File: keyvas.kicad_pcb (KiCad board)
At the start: 2 copper layers, 133 parts, among them J2 SWD, J3 USB-C Conn, J4 Conn_01x02_Female, K1 KEYSW, K10 KEYSW, K11 KEYSW, K12 KEYSW, K13 KEYSW, K14 KEYSW, K15 KEYSW, K16 KEYSW, K17 KEYSW, K18 KEYSW, K19 KEYSW, K2 KEYSW, K20 KEYSW, K21 KEYSW, K22 KEYSW, K23 KEYSW, K24 KEYSW, K25 KEYSW, K26 KEYSW, K27 KEYSW, K28 KEYSW, K29 KEYSW, K3 KEYSW, K30 KEYSW, K31 KEYSW, K32 KEYSW, K33 KEYSW, K34 KEYSW, K35 KEYSW, K36 KEYSW, K37 KEYSW, K38 KEYSW, K39 KEYSW, K4 KEYSW, K40 KEYSW, K41 KEYSW, K42 KEYSW, K43 KEYSW, K44 KEYSW, K45 KEYSW, K46 KEYSW, K47 KEYSW, K48 KEYSW, K5 KEYSW, K6 KEYSW, K7 KEYSW, K8 KEYSW, K9 KEYSW, Q2 AO3407, SW31 SW_SPDT, U2 XC6220B331MR-G, U3 TP4054, U4 USBLC6-2SC6, U5 E73-2G4M08S1C, X1 32.768kHz

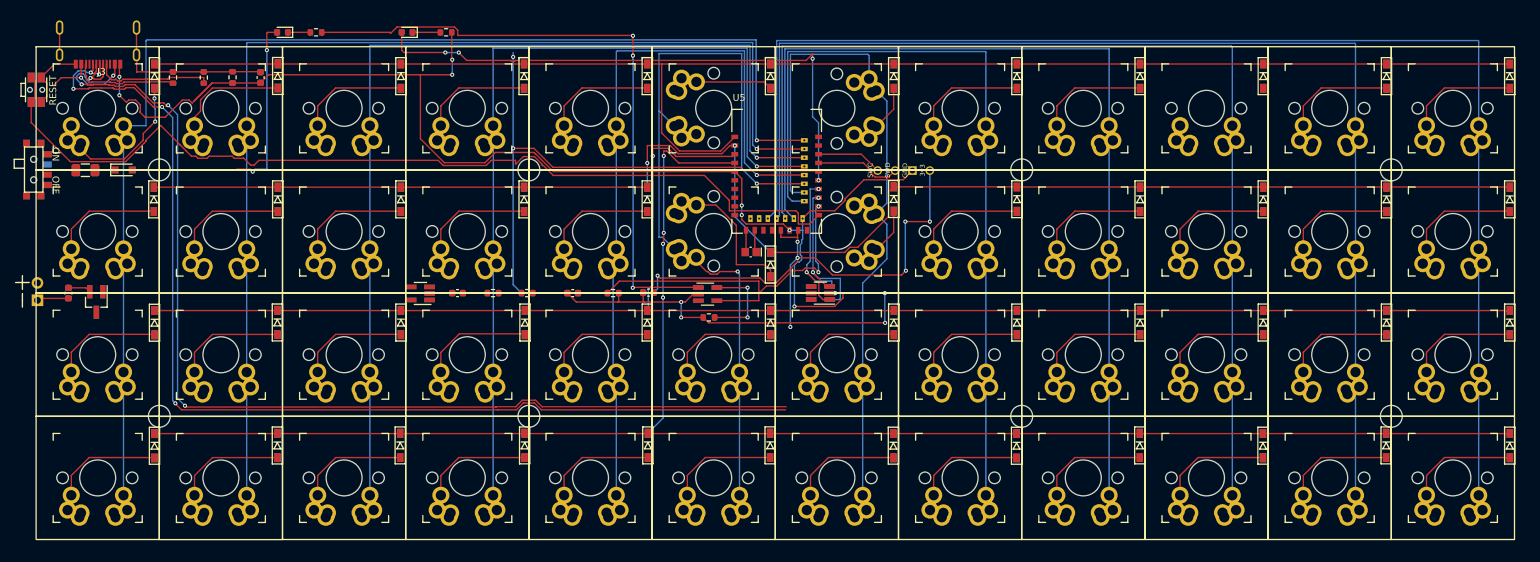
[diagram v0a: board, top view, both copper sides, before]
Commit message: finish
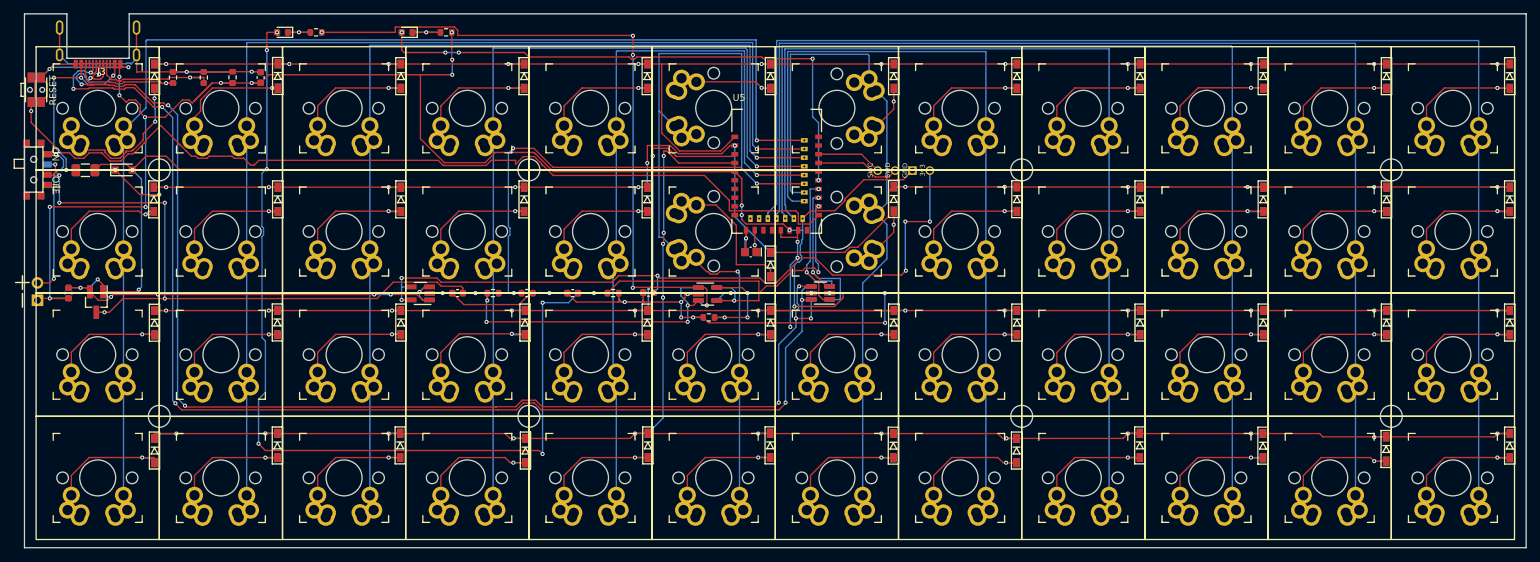
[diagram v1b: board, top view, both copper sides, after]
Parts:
- moved D43 0.76 mm to (107.5, 89.0)
- moved D40 0.70 mm to (53.3, 89.0)
- moved D47 0.70 mm to (179.2, 89.0)
- moved D50 0.53 mm to (233.2, 88.8)
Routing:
- net VBUS: track 90.4 -> 261.1 mm, vias 4 -> 14
- net VBAT: track 3.58 -> 148.3 mm, vias 0 -> 11
- net GND: track 277.5 -> 372.6 mm, vias 13 -> 27
- net Net-(D31-K): track 3.36 -> 86.8 mm, vias 0 -> 8
- net nRF_VDD: track 79.5 -> 123.8 mm, vias 7 -> 10
- net ROW2: track 234.8 -> 273.5 mm, vias 1 -> 13
- net Net-(J4-Pin_2): track 0.00 -> 25.0 mm, vias 0 -> 2
- net USBN: track 158.9 -> 183.2 mm, vias 4 -> 8
- net ROW3: track 252.0 -> 276.2 mm, vias 4 -> 16
- net GNDS: track 28.7 -> 51.4 mm, vias 0 -> 2
- net USBP: track 158.0 -> 178.9 mm, vias 5 -> 7
- net ROW0: track 220.7 -> 241.5 mm, vias 0 -> 12
- net ROW1: track 223.8 -> 242.6 mm, vias 2 -> 13
- net Net-(D10-A): track 0.00 -> 18.0 mm, vias 0 -> 1
- net Net-(F1-Pad1): track 14.0 -> 29.1 mm, vias 2 -> 4
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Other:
- board outline added: 219.4 x 78 mm
